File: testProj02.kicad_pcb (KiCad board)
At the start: 2 copper layers, 50 x 29 mm, 29 parts, among them J1 Conn_02x03_Odd_Even, J2 Conn_01x09_Pin, J3 Conn_01x04_Pin, J4 Conn_01x04_Pin, U1 24LC1025, U2 DS1337S_, U3 24LC1025, U4 ATMEGA328P-AU, Y1 32.768 KHZ, Y2 16 Mhz

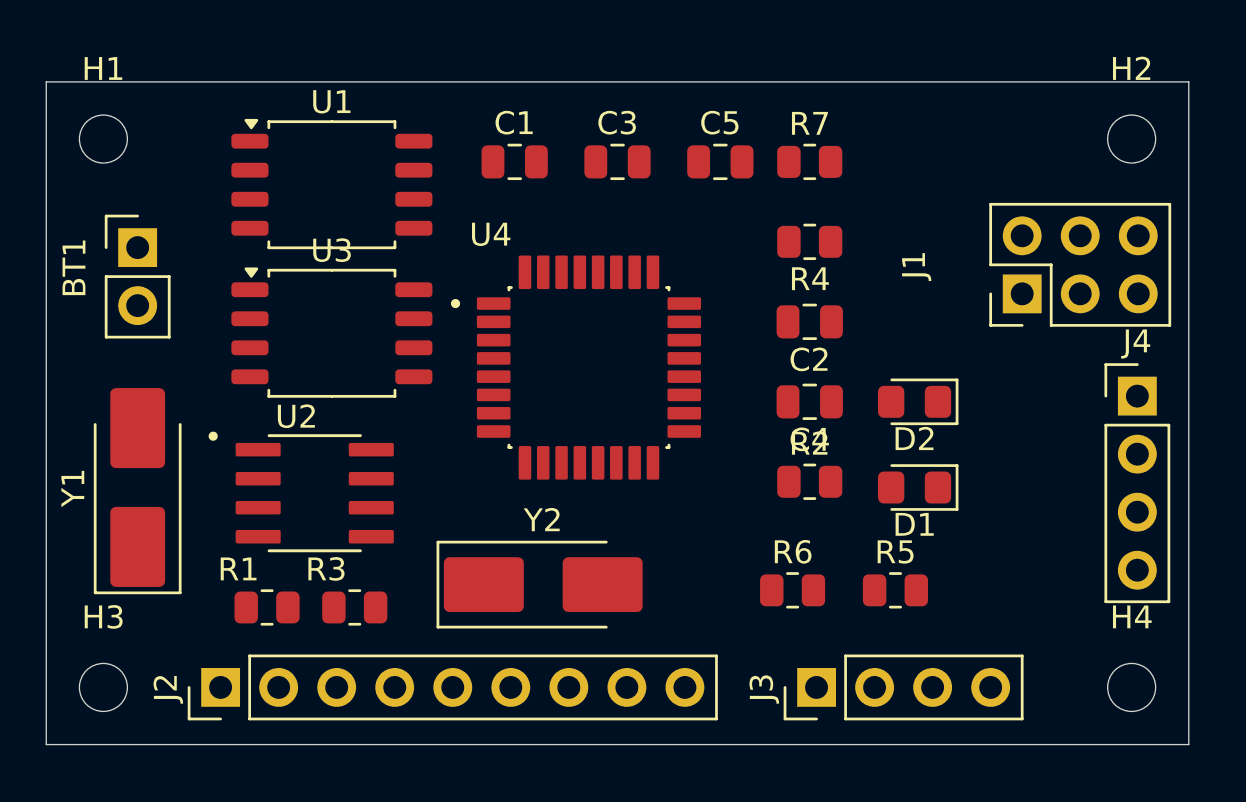
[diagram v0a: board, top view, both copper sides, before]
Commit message: test
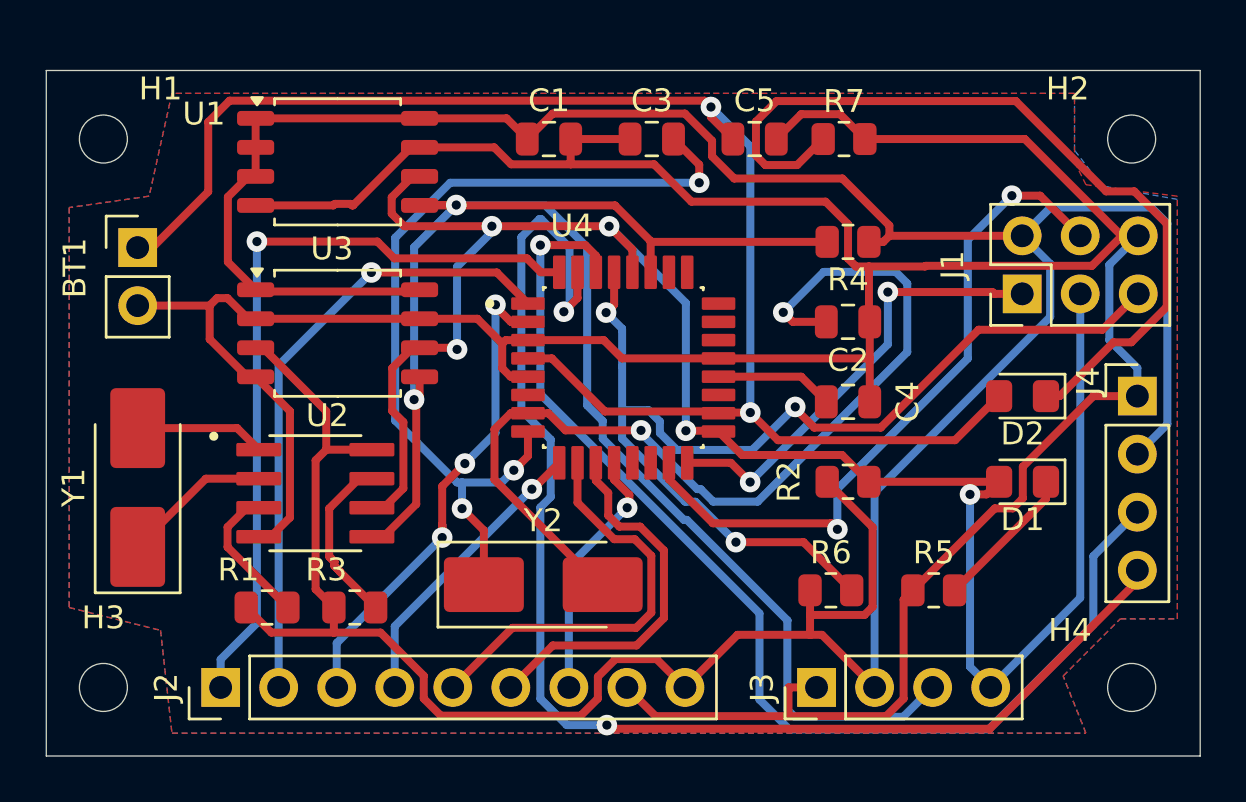
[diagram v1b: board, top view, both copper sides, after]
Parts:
- moved D1 4.73 mm to (104.7, 95.5)
- moved D2 4.73 mm to (104.7, 91.8)
- moved C1 1.80 mm to (84.0, 80.5)
- moved C3 1.80 mm to (88.5, 80.5)
- moved C5 1.80 mm to (93.0, 80.5)
- moved R7 1.80 mm to (96.9, 80.5)
- moved C2 1.68 mm to (97.1, 88.5)
- moved C4 1.68 mm to (97.1, 92.0)
- moved R2 1.68 mm to (97.1, 95.5)
- moved R4 1.68 mm to (97.1, 85.0)
- moved R5 1.68 mm to (100.8, 100.2)
- moved R6 1.68 mm to (96.3, 100.2)
- moved U4 1.50 mm to (87.2, 90.5)
- moved U1 1.03 mm to (74.8, 81.5)
- moved U3 0.25 mm to (74.8, 89.0)
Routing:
- net GND: track 0.00 -> 162.2 mm
- net /Vcc: track 0.00 -> 157.1 mm
- net /SCK: track 0.00 -> 86.0 mm, vias 0 -> 5
- net /SDA: track 0.00 -> 76.5 mm, vias 0 -> 2
- net Net-(BT1-+): track 0.00 -> 68.5 mm, vias 0 -> 2
- net /TX: track 0.00 -> 58.6 mm, vias 0 -> 2
- net /RX: track 0.00 -> 50.0 mm, vias 0 -> 1
- net /RESET: track 0.00 -> 49.9 mm, vias 0 -> 3
- net Net-(U4-PB6): track 0.00 -> 43.0 mm, vias 0 -> 2
- net Net-(U4-PB7): track 0.00 -> 41.0 mm, vias 0 -> 3
- net Net-(D2-K): track 0.00 -> 36.2 mm
- net /D2: track 0.00 -> 34.0 mm, vias 0 -> 1
- net /MOSI: track 0.00 -> 32.0 mm, vias 0 -> 2
- net /D3: track 0.00 -> 27.3 mm, vias 0 -> 1
- net /D4: track 0.00 -> 23.9 mm, vias 0 -> 3
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- added copper zone on B.Cu, net GND
- added copper zone on F.Cu, net GND
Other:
- board size 50 x 29 mm -> 50.5 x 30 mm
